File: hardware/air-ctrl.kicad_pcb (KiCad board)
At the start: 2 copper layers, 35 x 35 mm, 67 parts, among them J1 USB_C_Receptacle_USB2.0_16P, J2 SFV24R-2STE1HLF, J3 Conn_ARM_SWD_TagConnect_TC203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, J4 Conn_01x02, Q1 BSS138, SW1 SW_RST, U1 nRF52832-QFxx, U2 BME688, U3 MCP73871-2CC, U4 MCP1700x-330xxTT, U5 USBLC6-2SC6, Y1 32MHz, Y2 32.768kHz

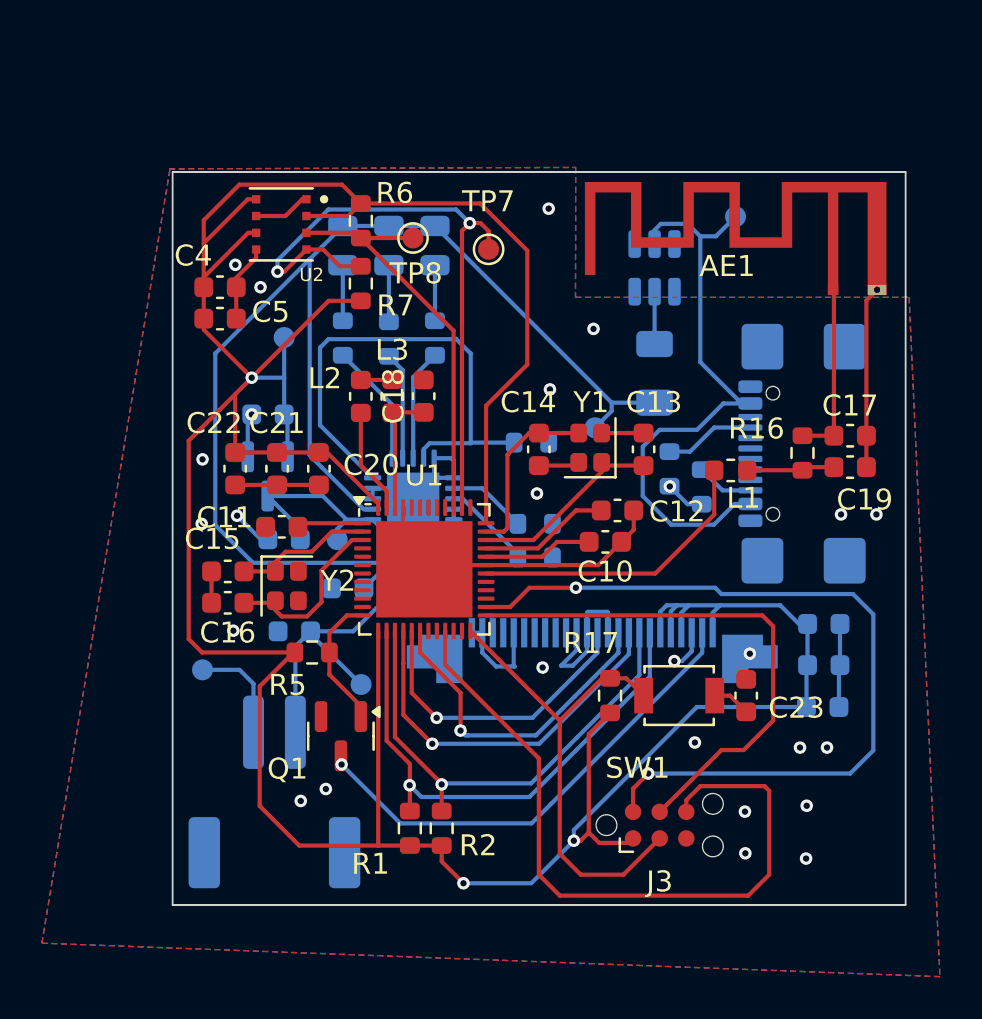
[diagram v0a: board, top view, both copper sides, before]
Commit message: fixed antenna layout
wip: placing components
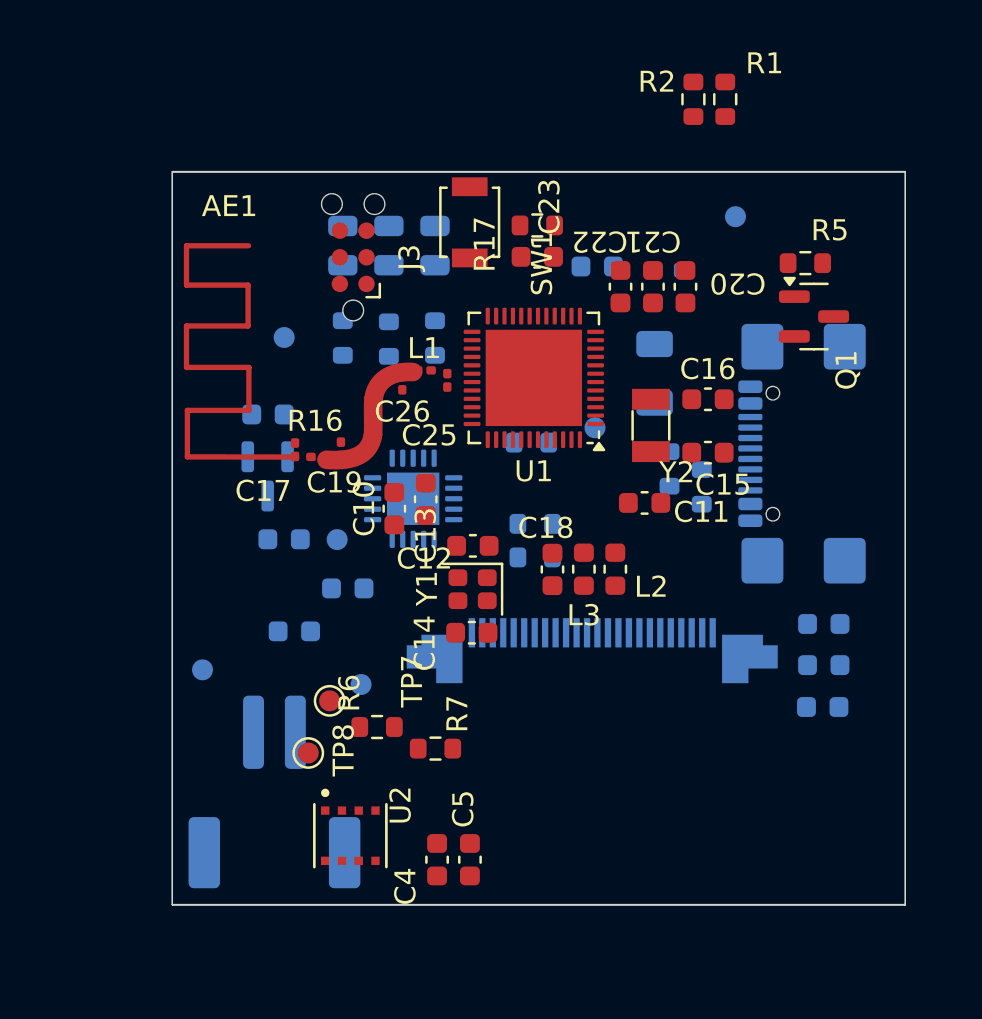
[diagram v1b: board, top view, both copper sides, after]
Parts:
- removed U5: USBLC6-2SC6, Package_TO_SOT_SMD:SOT-23-6
- added C24: 100nF, Capacitor_SMD:C_0603_1608Metric, B.Cu at (170.3, 44.5)
- added C25: 0.8pF, Capacitor_SMD:C_0201_0603Metric, F.Cu at (163.1, 49.9)
- added C26: NC, Capacitor_SMD:C_0201_0603Metric, F.Cu at (161.0, 50.1)
- added D4: ESD5Zxx, Diode_SMD:D_SOD-523, B.Cu at (173.6, 44.7)
- AE1: value BLE -> ~; footprint RF_Antenna:Texas_SWRA117D_2.4GHz_Left -> RF_Antenna:Antenna_BLE
- C17: value 0.8pF -> 1.5pF; footprint Capacitor_SMD:C_0603_1608Metric -> Capacitor_SMD:C_0201_0603Metric
- C19: value 0.8pF -> 0.5pF; footprint Capacitor_SMD:C_0603_1608Metric -> Capacitor_SMD:C_0201_0603Metric
- L1: value 3.9nH -> 4.7nH; footprint Inductor_SMD:L_0603_1608Metric -> Inductor_SMD:L_0201_0603Metric
- R16: footprint Resistor_SMD:R_0603_1608Metric -> Resistor_SMD:R_0201_0603Metric
- Y2: footprint Crystal:Crystal_SMD_2016-4Pin_2.0x1.6mm -> Crystal:Crystal_SMD_3215-2Pin_3.2x1.5mm
- moved R1 37.9 mm to (176.4, 36.5), turned to -90 degrees
- moved R2 36.8 mm to (174.9, 36.5), turned to -90 degrees
- moved J3 30.8 mm to (158.6, 44.1), turned to 90 degrees
- moved Q1 30.2 mm to (180.6, 46.9), turned to 0 degrees
- moved R5 30.0 mm to (180.2, 44.4), turned to 180 degrees
- moved U2 29.4 mm to (158.5, 71.7), turned to 90 degrees
- moved C4 29.2 mm to (162.6, 72.8), turned to 90 degrees
- moved C5 28.5 mm to (164.2, 72.8), turned to 90 degrees
- moved AE1 28.1 mm to (153.7, 48.8), turned to 90 degrees
- moved C17 26.5 mm to (155.9, 53.3), turned to 90 degrees
- moved TP8 25.1 mm to (156.5, 67.7), turned to 90 degrees
- moved C16 24.9 mm to (175.6, 50.9), turned to 0 degrees
- moved SW1 24.7 mm to (164.2, 42.4), turned to -90 degrees
- moved C19 24.3 mm to (158.1, 53.2), turned to 90 degrees
- moved R6 24.2 mm to (159.8, 66.5), turned to 0 degrees
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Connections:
- C23 pad 1: Net-(C23-Pad1) -> -BATT
- C23 pad 2: -BATT -> Net-(J3-~{RESET})
- F1 pad 1: Net-(U5-GND) -> /power/V_BUS
- SW1 pad 1: Net-(C23-Pad1) -> -BATT
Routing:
- net /power/V_3V3: track 170.2 -> 0.00 mm, vias 3 -> 0
- net -BATT: track 76.3 -> 0.00 mm, vias 26 -> 0
- net /power/V_IN: track 66.2 -> 0.00 mm
- net Net-(J3-SWDIO): track 39.2 -> 0.00 mm, vias 2 -> 0
- net Net-(J3-SWO): track 34.2 -> 0.00 mm
- net /mcu/I2C_SCL: track 31.4 -> 0.00 mm, vias 2 -> 0
- net /power/V_BUS: track 29.0 -> 0.00 mm
- net Net-(J3-SWCLK): track 25.7 -> 0.00 mm
- net /display/DISP_RST: track 25.2 -> 0.00 mm, vias 1 -> 0
- net Net-(U3-THERM): track 24.1 -> 0.00 mm
- net Net-(J3-~{RESET}): track 23.5 -> 0.00 mm
- net /display/DISP_CS: track 23.2 -> 0.00 mm, vias 1 -> 0
- net /display/LEDK: track 22.7 -> 0.00 mm, vias 1 -> 0
- net /mcu/I2C_SDA: track 19.9 -> 0.00 mm
- net +BATT: track 18.5 -> 0.00 mm
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- removed copper zone on B.Cu, net -BATT
- removed copper zone on F.Cu, net -BATT
